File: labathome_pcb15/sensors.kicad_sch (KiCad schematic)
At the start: 23 parts, among them J12 TCS34725, J16 BMEx80, J19 BH1750, J20 CCS811, J21 QWIIC, J23 VL53L5x, J4 SCD4x, U12 AHT20, U14 BMP280, U19 DS18B20, U22 AM612, U7 DS18B20, U9 LSM6DS3

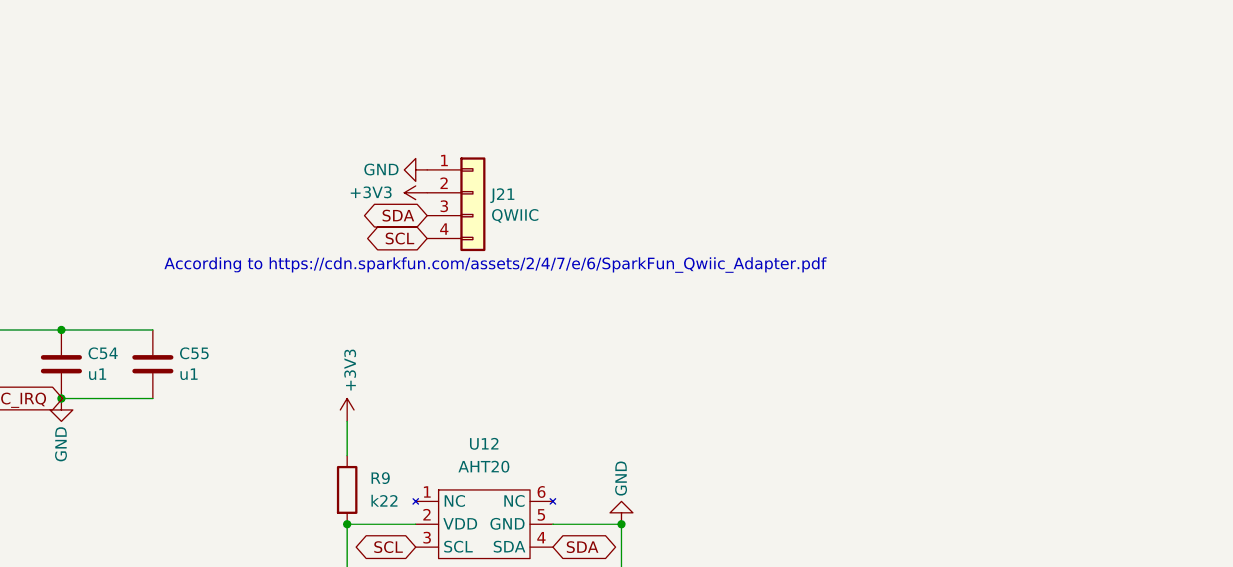
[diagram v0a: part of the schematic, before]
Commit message: lbathome 15.1
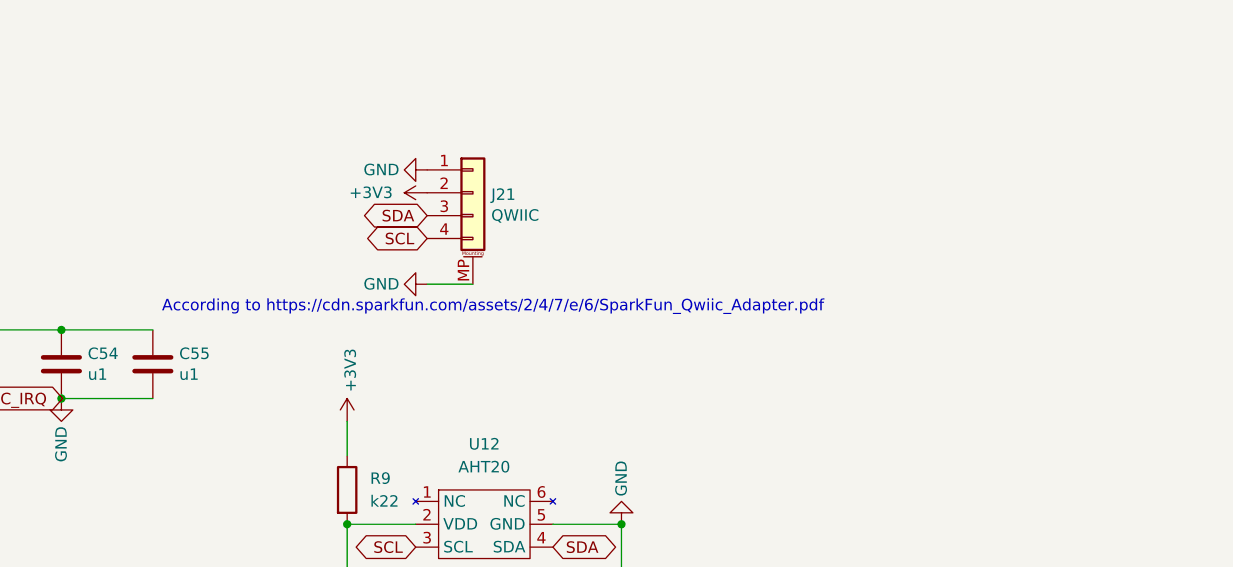
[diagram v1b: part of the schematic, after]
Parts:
- J21: symbol Connector_Generic:Conn_01x04 -> Connector_Generic_MountingPin:Conn_01x04_MountingPin
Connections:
- net GND: now also J21.MP (MountPin)
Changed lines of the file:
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@@
 	(wire
 		(pts
+			(xy 137.16 95.25) (xy 142.24 95.25)
+		)
+		(stroke
+			(width 0)
+			(type default)
+		)
+	)
+	(wire
+		(pts
 			(xy 158.75 121.92) (xy 158.75 129.54)
 		)
@@
 	(text "According to https://cdn.sparkfun.com/assets/2/4/7/e/6/SparkFun_Qwiic_Adapter.pdf"
 		(exclude_from_sim no)
-		(at 107.95 93.98 0)
+		(at 107.696 98.552 0)
 		(effects
 			(font
@@
 	)
 	(symbol
-		(lib_id "Connector_Generic:Conn_01x04")
+		(lib_id "Connector_Generic_MountingPin:Conn_01x04_MountingPin")
 		(at 142.24 85.09 0)
 		(unit 1)
@@
 			)
 		)
-		(property "Description" ""
+		(property "Description" "Generic connectable mounting pin connector, single row, 01x04, script generated (kicad-library-utils/schlib/autogen/connector/)"
 			(at 142.24 85.09 0)
 			(effects
@@
 		(pin "4"
 		)
+		(pin "MP"
+		)
 		(instances
 			(project "pcbV10"
@@
 					(unit 1)
 				)
+			)
+		)
+	)
+	(symbol
+		(lib_id "power:GND")
+		(at 137.16 95.25 270)
+		(unit 1)
+		(exclude_from_sim no)
+		(in_bom yes)
+		(on_board yes)
+		(dnp no)
+		(property "Reference" "#PWR038"
+			(at 130.81 95.25 0)
+			(effects
+				(font
+					(size 1.27 1.27)
+				)
+				(hide yes)
+			)
+		)
+		(property "Value" "GND"
+			(at 132.08 95.25 90)
+			(effects
+				(font
+					(size 1.27 1.27)
+				)
+			)
+		)
+		(property "Footprint" ""
+			(at 137.16 95.25 0)
+			(effects
+				(font
+					(size 1.27 1.27)
+				)
+				(hide yes)
+			)
+		)
+		(property "Datasheet" ""
+			(at 137.16 95.25 0)
+			(effects
+				(font
+					(size 1.27 1.27)
+				)
+				(hide yes)
+			)
+		)
+		(property "Description" "Power symbol creates a global label with name \"GND\" , ground"
+			(at 137.16 95.25 0)
+			(effects
+				(font
+					(size 1.27 1.27)
+				)
+				(hide yes)
+			)
+		)
+		(pin "1"
+		)
+		(instances
+			(project "labathome_pcb15"
+				(path "/e4d6926a-1a8b-424d-97c4-66b6ad87e4ac/faeff10d-104f-4ca8-a480-26bd51140cf0"
+					(reference "#PWR038")
+					(unit 1)
+				)
